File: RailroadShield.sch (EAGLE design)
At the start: 39 parts, among them J1 I2C, J4 MST4V, J5 RJ12, J6 RJ12, Q1 2N3904, U1 LM393N, U2 MCP2515-P, U3 MCP2551-P, Y1 RESONATORPTH

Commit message: 1.1
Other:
- note added: "1.1"
- note removed: "1.0"
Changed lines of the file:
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@@
 <text x="43.18" y="149.86" size="1.27" layer="250">Termination</text>
 <text x="149.86" y="27.94" size="5.08" layer="250">Locoduino</text>
-<text x="238.76" y="7.62" size="2.54" layer="250">1.0</text>
+<text x="238.76" y="7.62" size="2.54" layer="250">1.1</text>
 <text x="155.194" y="24.13" size="2.54" layer="250">Control Point</text>
 <text x="195.58" y="27.94" size="2.54" layer="250">Loconet &amp; CAN/NMRAnet</text>

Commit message: 1.2
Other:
- note added: "1.2"
- note removed: "1.1"
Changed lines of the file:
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@@
 <text x="43.18" y="149.86" size="1.27" layer="250">Termination</text>
 <text x="149.86" y="27.94" size="5.08" layer="250">Locoduino</text>
-<text x="238.76" y="7.62" size="2.54" layer="250">1.1</text>
+<text x="238.76" y="7.62" size="2.54" layer="250">1.2</text>
 <text x="155.194" y="24.13" size="2.54" layer="250">Control Point</text>
 <text x="195.58" y="27.94" size="2.54" layer="250">Loconet &amp; CAN/NMRAnet</text>

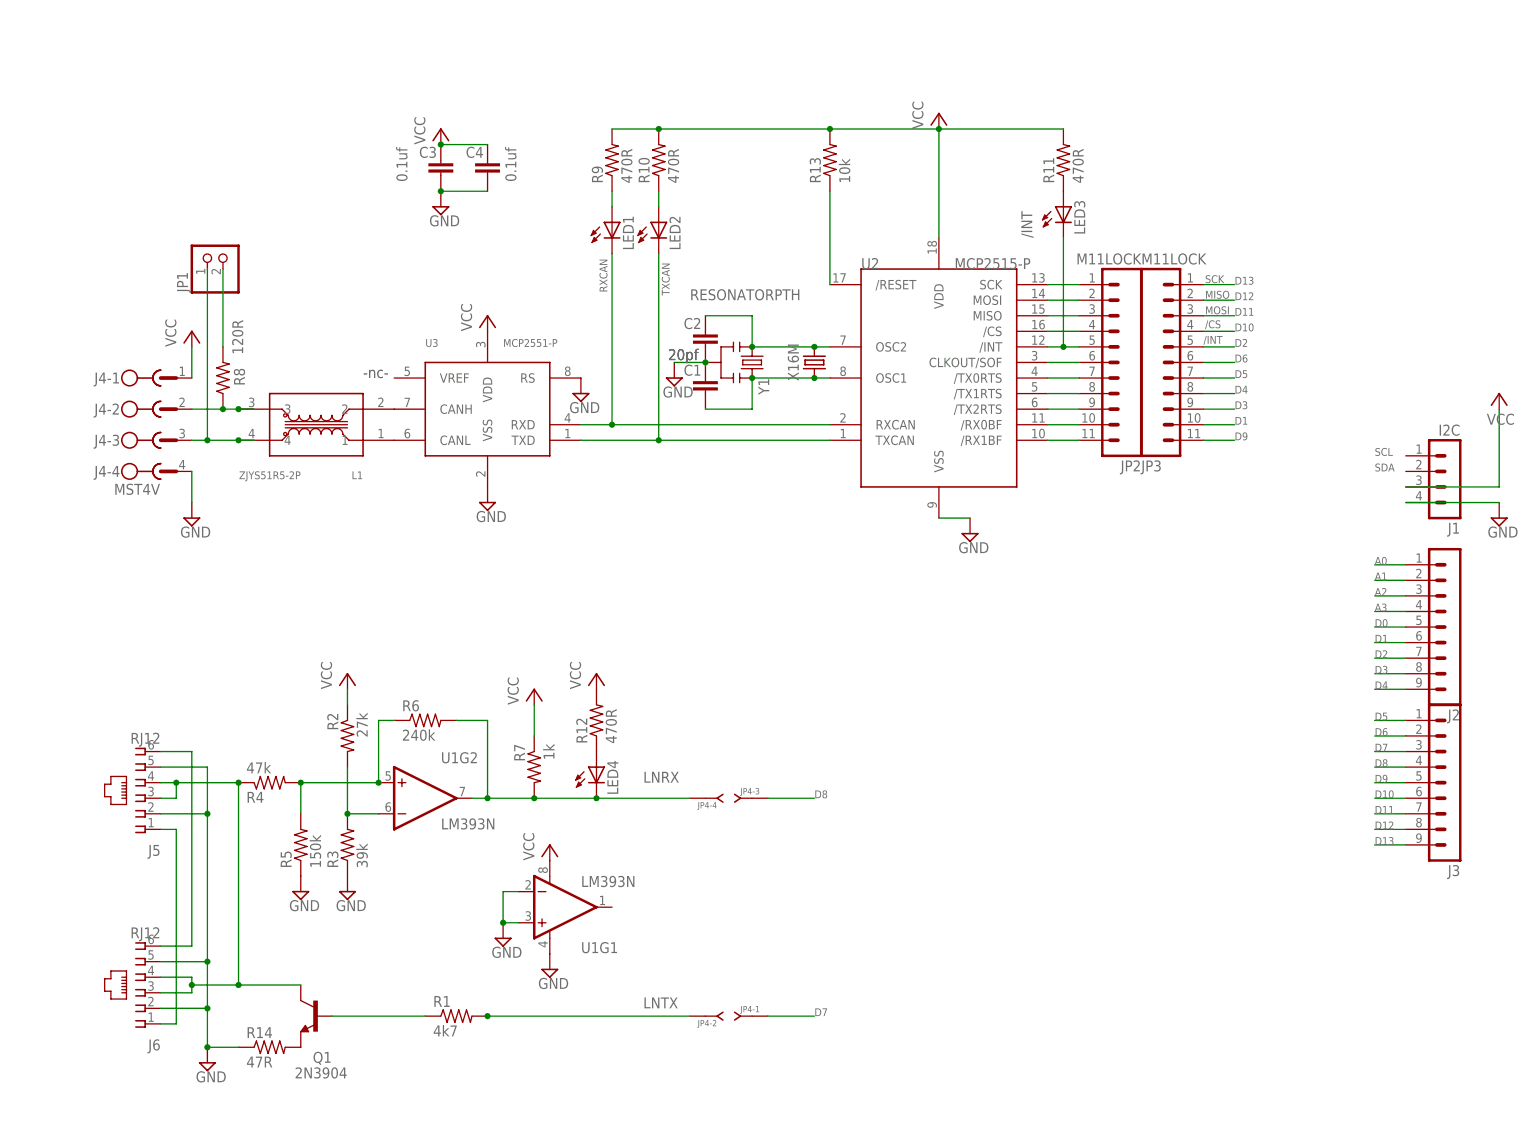
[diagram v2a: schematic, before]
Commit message: 1.3
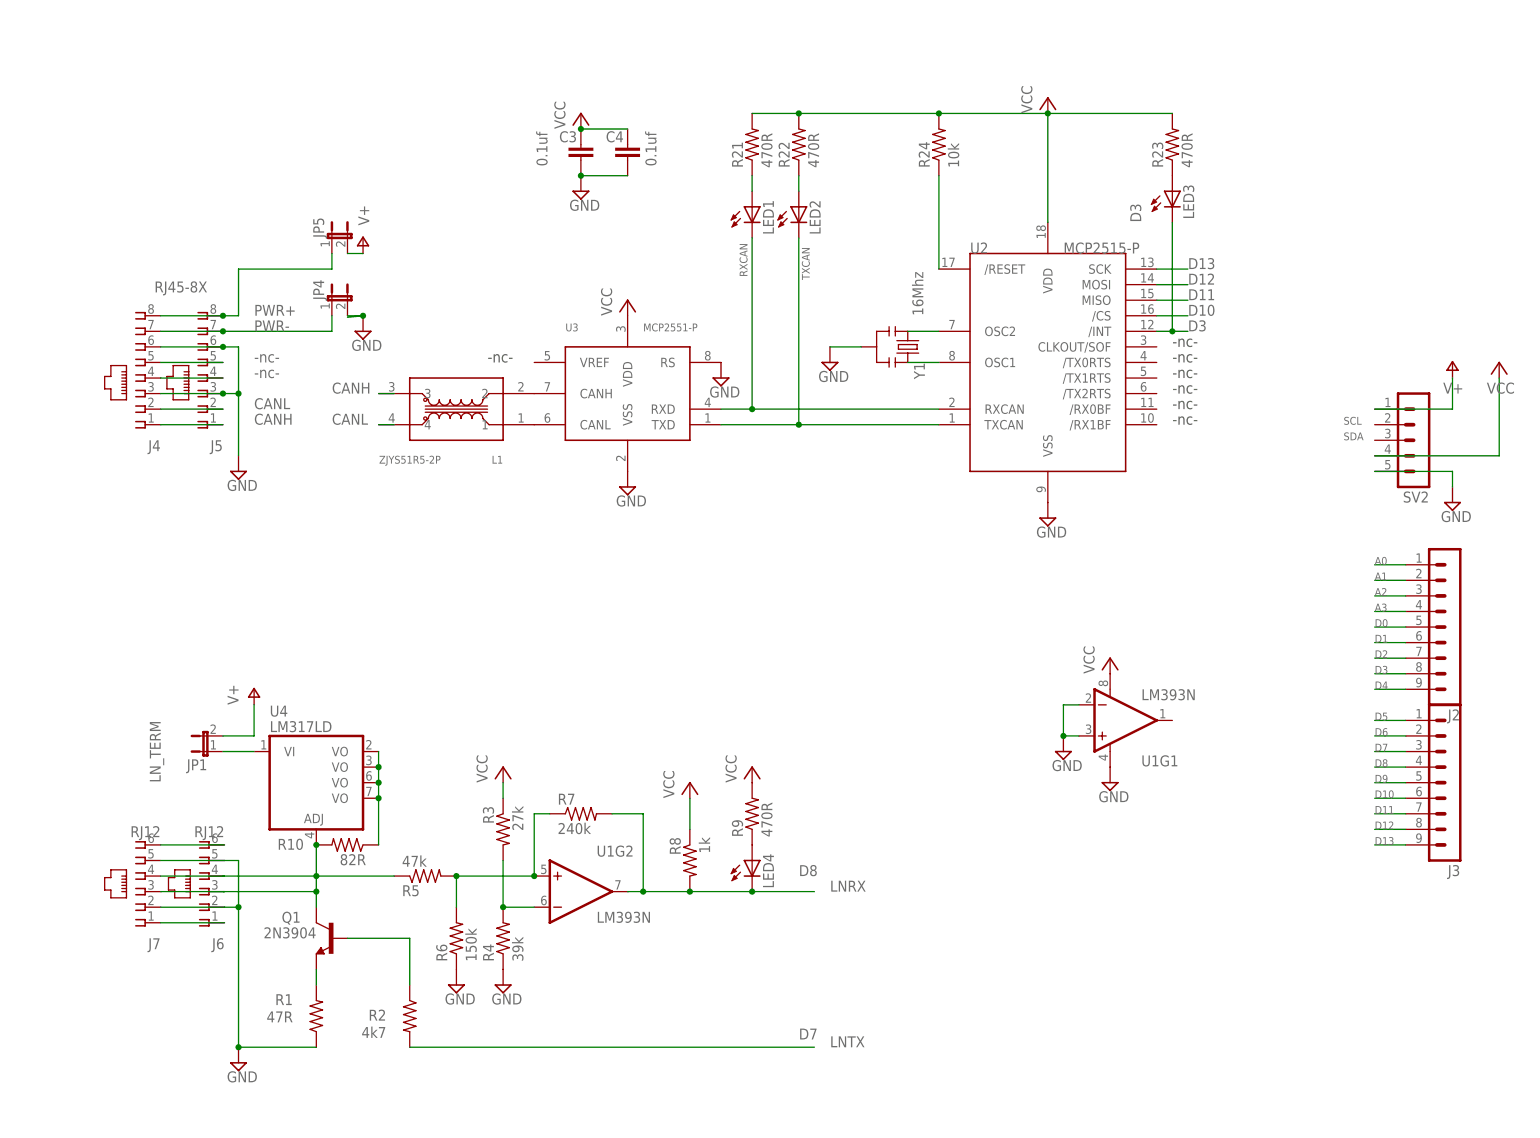
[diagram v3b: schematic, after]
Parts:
- removed C1, C2: 20pf, SparkFun:CAP0603-CAP
- removed J1: I2C, con-lstb:MA04-1
- removed JP2, JP3: M11LOCK, SparkFun:M11LOCK
- removed R11, R12: 470R, rcl:R-US_R1206W
- removed R13: 10k, rcl:R-US_R1206W
- removed R14: 47R, rcl:R-US_R1206W
- removed X16M: (no value), crystal:CRYSTALHC49S
- added J7: RJ12, con-amp:520250-3
- added JP5: (no value), SparkFun:JUMPER-2PTH_LOCK
- added R21, R22, R23: 470R, rcl:R-US_R1206W
- added R24: 10k, rcl:R-US_R1206W
- added SV2: (no value), con-lstb:MA05-1
- added U4: LM317LD, linear:LM317LD
- J4: value MST4V -> RJ45-8X; device con-phoenix-508:MST4V -> con-tycoelectronics:RJ45-8X
- J5: value RJ12 -> RJ45-8X; device con-amp:520250-3 -> con-tycoelectronics:RJ45-8X
- JP1: device pinhead:PINHD-1X2 -> SparkFun:JUMPER-2PTH
- JP4: value J-04-100-2X02 -> (none); device con-headers-jp:J-04-100-2X02 -> SparkFun:JUMPER-2PTH_LOCK
- R1: value 4k7 -> 47R
- R10: value 470R -> 82R
- R2: value 27k -> 4k7
- R3: value 39k -> 27k
- R4: value 47k -> 39k
- R5: value 150k -> 47k
- R6: value 240k -> 150k
- R7: value 1k -> 240k
- R8: value 120R -> 1k
- Y1: value RESONATORPTH -> 16Mhz
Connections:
- removed net /INT: JP2.5, LED3.C, U2./INT
- removed net /RX0BF: JP2.10, U2./RX0BF
- removed net /RX1BF: JP2.11, U2./RX1BF
- removed net /TX0RTS: JP2.7, U2./TX0RTS
- removed net /TX1RTS: JP2.8, U2./TX1RTS
- removed net /TX2RTS: JP2.9, U2./TX2RTS
- removed net CLKOUT: JP2.6, U2.CLKOUT/SOF
- removed net DCCRAILSYNC-: J5.1, J6.1
- removed net LNRX: JP4-4.J, LED4.C, R6.2, R7.2, U1G2.OUT
- removed net LNTX: JP4-2.J, R1.2
- removed net N$20: JP2.4, U2./CS
- removed net OSC2: C2.1, U2.OSC2, X16M.2, Y1.1
- removed net RAILSYNC+: J5.6, J6.6
- new net CANH: J4.1, J5.1, L1.3
- new net CANL: J4.2, J5.2, L1.4
- new net N$17: R10.1, U4.VO, U4.VO@1, U4.VO@2, U4.VO@3
- new net N$18: J4.4, J5.4
- new net N$21: J4.5, J5.5
- new net PWR+: J4.8, J5.8, JP5.1
- new net PWR-: J4.7, J5.7, JP4.1
- new net V+: JP1.2, JP5.2, SV2.1
- net /RESET: now also R24.1; no longer R13.1
- net D1: no longer JP3.10
- net D10: now also U2./CS; no longer JP3.4
- net D11: now also U2.MISO; no longer JP3.3
- net D12: now also U2.MOSI; no longer JP3.2
- net D13: now also U2.SCK; no longer JP3.1
- net D2: no longer JP3.5
- net D3: now also LED3.C, U2./INT; no longer JP3.9
- net D4: no longer JP3.8
- net D5: no longer JP3.7
- net D6: no longer JP3.6
- net D7: now also R2.2; no longer JP4-1.J
- net D8: now also LED4.C, R7.2, R8.2, U1G2.OUT; no longer JP4-3.J
- net D9: no longer JP3.11
- net GND: now also J4.3, J4.6, J5.3, J5.6, J7.2, J7.5, JP4.2, R1.1, R4.1, R6.1, SV2.5; no longer C1.1, C2.2, J1.4, J4-4.1, J5.2, J5.5, R14.1, R3.1, R5.1
- net LOCONET: now also R10.2, R5.1, U4.ADJ; no longer J5.3, J5.4, J6.3, J6.4, R4.1
- net N$1: now also R2.1; no longer R1.1
- net N$10: now also J6.6, J7.6; no longer JP1.2, R8.2
- net N$11: now also R21.1; no longer R9.1
- net N$12: now also R22.1; no longer R10.1
- net N$13: now also J6.3, J7.3; no longer JP2.1, U2.SCK
- net N$14: now also R23.1; no longer R11.1
- net N$15: now also R9.1; no longer R12.1
- net N$16: now also J6.4, J7.4; no longer JP2.2, U2.MOSI
- net N$19: now also JP1.1, U4.VI; no longer JP2.3, U2.MISO
- net N$2: now also R6.2, R7.1; no longer R4.2, R6.1
- net N$5: now also R4.2; no longer R2.2
- net N$6: now also R1.2; no longer R14.2
- net N$8: now also U2.OSC2, Y1.1; no longer J4-2.1, L1.3, R8.1
- net N$9: now also J6.1, J7.1; no longer J4-3.1, JP1.1, L1.4
- net OSC1: no longer C1.2, X16M.1
- net VCC: now also R21.2, R22.2, R23.2, R24.2, R3.1, R8.1, SV2.4; no longer J1.3, J4-1.1, R10.2, R11.2, R12.2, R13.2, R2.1, R7.1
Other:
- note added: "1.3"
- note added: "LNRX"
- note added: "LNTX"
- note added: "LN_TERM"
- note removed: "/CS"
- note removed: "/INT"
- note removed: "1.2"
- note removed: "MISO"
- note removed: "MOSI"
- note removed: "SCK"
- note removed: "Termination"
- moved on the sheet: C3, C4, J6, L1, LED1, LED2, LED3, LED4, Q1, R1, R10, R2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

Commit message: 2.0
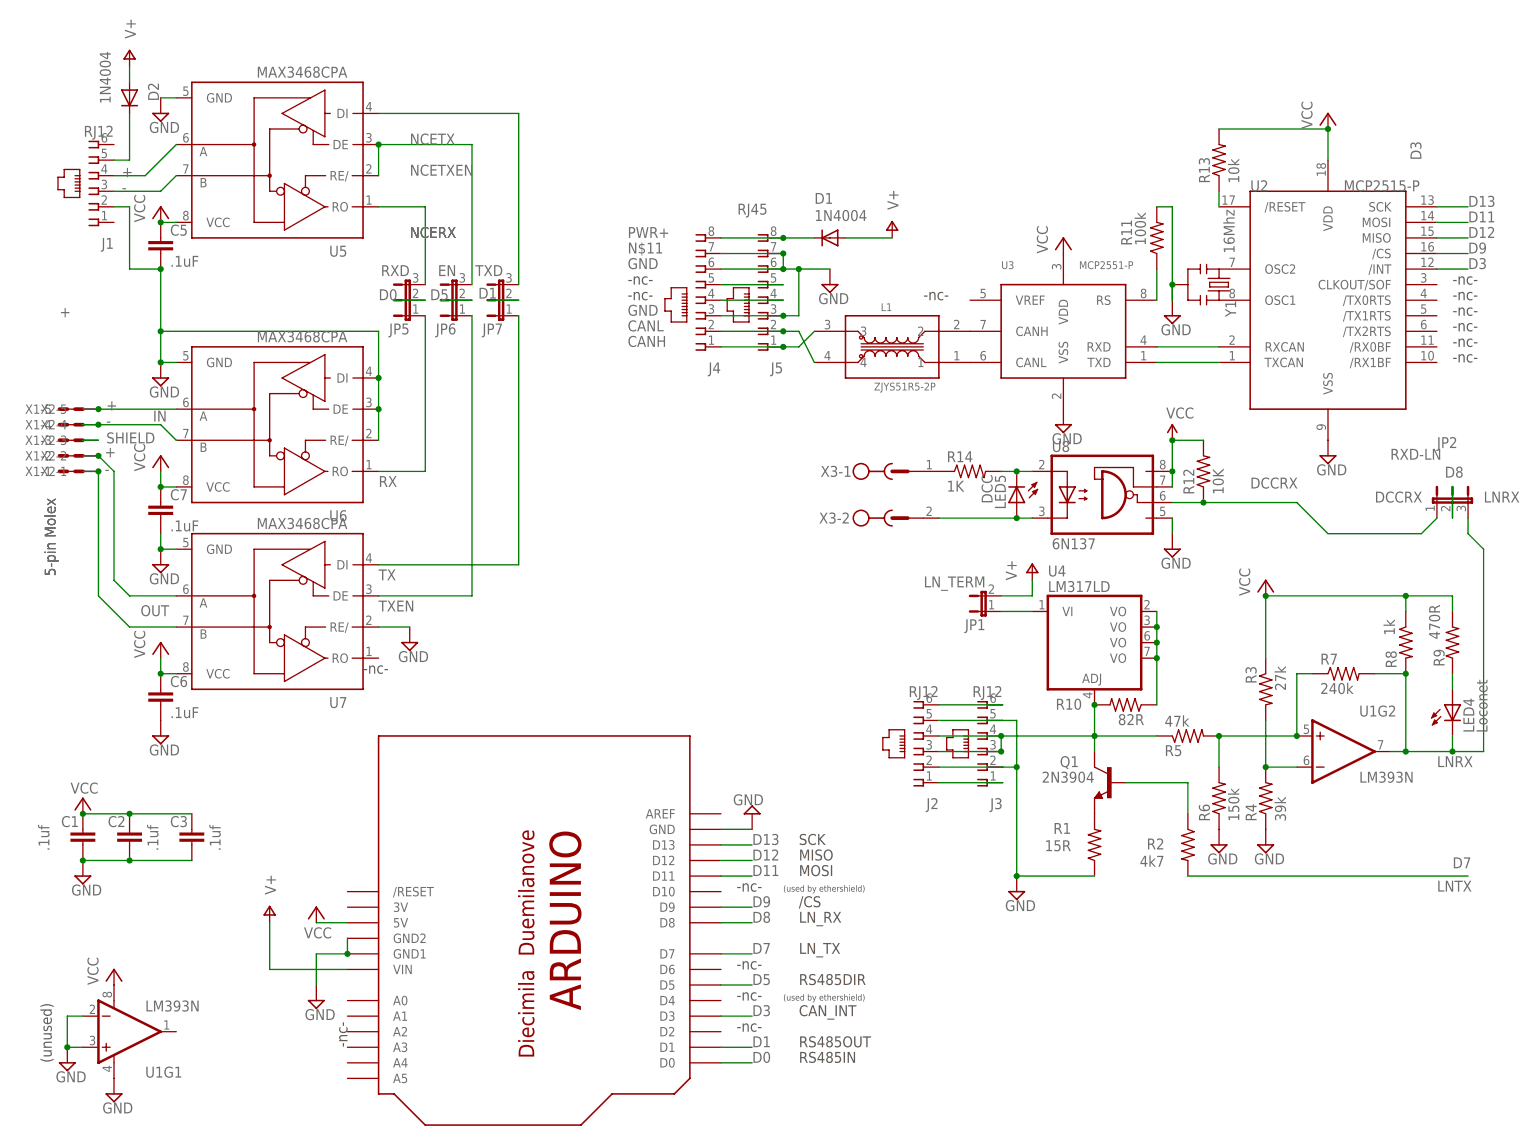
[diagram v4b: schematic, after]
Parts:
- removed C4: 0.1uf, SparkFun:CAPPTH2
- removed J6, J7: RJ12, con-amp:520250-3
- removed JP4: (no value), SparkFun:JUMPER-2PTH_LOCK
- removed LED1, LED2, LED3: (no value), MCP:LEDB155
- removed R21, R22, R23: 470R, rcl:R-US_R1206W
- removed R24: 10k, rcl:R-US_R1206W
- removed SV2: (no value), con-lstb:MA05-1
- added C1, C2: .1uf, SparkFun:CAPPTH2
- added C5, C6, C7: .1uF, SparkFun:CAPPTH2
- added D1, D2: 1N4004, diode:1N4004
- added J1: RJ12, con-amp:520250-3
- added JP2: RXD-LN, SparkFun:JUMPER-3PTH
- added JP6: EN, SparkFun:JUMPER-3PTH
- added JP7: TXD, SparkFun:JUMPER-3PTH
- added LED5: DCC, MCP:LEDCHIP-LED0805
- added MOD1: ARDUINO DUEMILANOVE, microbuilder:ARDUINODUEMILANOVE
- added R11: 100k, rcl:R-US_R1206
- added R12: 10K, SparkFun:RESISTOR1206
- added R13: 10k, rcl:R-US_R1206
- added R14: 1K, SparkFun:RESISTOR1206
- added U5, U6, U7: MAX3468CPA, maxim:MAX3468CPA
- added U8: 6N137, optocoupler:6N137
- added X1, X2: 5-pin Molex, con-molex:KK-156-5
- added X3: (no value), con-phoenix-500:MSTBV2
- C3: value 0.1uf -> .1uf
- J2, J3: value (none) -> RJ12; device con-lstb:MA09-1 -> con-amp:520250-3
- J4, J5: value RJ45-8X -> RJ45
- JP1: value (none) -> LN_TERM
- JP5: value (none) -> RXD; device SparkFun:JUMPER-2PTH_LOCK -> SparkFun:JUMPER-3PTH
- LED4: value (none) -> Loconet; device MCP:LEDB155 -> MCP:LEDCHIP-LED0805
- R1: value 47R -> 15R; device rcl:R-US_R1206W -> rcl:R-US_R1206
- R10, R2, R3, R4, R5, R6, R7, R8, R9: device rcl:R-US_R1206W -> rcl:R-US_R1206
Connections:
- removed net A0: J2.1
- removed net A1: J2.2
- removed net A2: J2.3
- removed net A3: J2.4
- removed net D10: J3.6, U2./CS
- removed net D2: J2.7
- removed net D4: J2.9
- removed net D6: J3.2
- removed net N$12: LED2.A, R22.1
- removed net N$14: LED3.A, R23.1
- removed net PWR-: J4.7, J5.7, JP4.1
- new net -OUT+: U7.B, X1-1.S, X2-1.S
- new net CMRIRX: JP5.1, U6.RO
- new net CMRITX: JP7.1, U7.DI
- new net CMRITXEN: JP6.1, U7.DE
- new net DCCRX: JP2.1, R12.1, U8.VO
- new net IN+: U6.A, X1-5.S, X2-5.S
- new net IN-: U6.B, X1-4.S, X2-4.S
- new net LNRX: JP2.3, LED4.C, R7.2, R8.2, U1G2.OUT
- new net N$20: R14.1, X3-1.SK
- new net N$23: J2.3, J3.3
- new net N$24: J1.4, U5.A
- new net N$25: J1.3, U5.B
- new net N$26: D2.C, J1.5
- new net N$4: R11.1, U3.RS
- new net NCERX: JP5.3, U5.RO
- new net NCETX: JP7.3, U5.DI
- new net NCETXEN: JP6.3, U5.DE, U5.RE/
- new net OUT+: U7.A, X1-2.S, X2-2.S
- new net SHIELD: X1-3.S, X2-3.S
- net /RESET: now also R13.1; no longer R24.1
- net D0: now also JP5.2, MOD1.D0; no longer J2.5
- net D1: now also JP7.2, MOD1.D1; no longer J2.6
- net D11: now also MOD1.D11, U2.MOSI; no longer J3.7, U2.MISO
- net D12: now also MOD1.D12, U2.MISO; no longer J3.8, U2.MOSI
- net D13: now also MOD1.D13; no longer J3.9
- net D3: now also MOD1.D3; no longer J2.8, LED3.C
- net D5: now also JP6.2, MOD1.D5; no longer J3.1
- net D7: now also MOD1.D7; no longer J3.3
- net D8: now also JP2.2, MOD1.D8; no longer J3.4, LED4.C, R7.2, R8.2, U1G2.OUT
- net D9: now also MOD1.D9, U2./CS; no longer J3.5
- net GND: now also C1.2, C2.2, C5.2, C6.2, C7.2, J1.2, J2.2, J2.5, J3.2, J3.5, MOD1.GND, MOD1.GND1, MOD1.GND2, R11.2, U5.GND, U6.DE, U6.DI, U6.GND, U6.RE/, U7.GND, U7.RE/, U8.GND; no longer C4.2, J6.2, J6.5, J7.2, J7.5, JP4.2, SV2.5, U3.RS
- net LOCONET: now also J2.4, J3.4
- net N$10: now also J2.6, J3.6; no longer J6.6, J7.6
- net N$11: now also J4.7, J5.7; no longer LED1.A, R21.1
- net N$13: now also LED5.A, U8.C, X3-2.SK; no longer J6.3, J7.3
- net N$16: now also LED5.C, R14.2, U8.A; no longer J6.4, J7.4
- net N$9: now also J2.1, J3.1; no longer J6.1, J7.1
- net PWR+: now also D1.C; no longer JP5.1
- net RXCAN: no longer LED1.C
- net TXCAN: no longer LED2.C
- net V+: now also D1.A, D2.A, MOD1.VIN; no longer JP5.2, SV2.1
- net VCC: now also C1.1, C2.1, C5.1, C6.1, C7.1, MOD1.5V, R12.2, R13.2, U5.VCC, U6.VCC, U7.VCC, U8.VCC, U8.VE; no longer C4.1, R21.2, R22.2, R23.2, R24.2, SV2.4
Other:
- note added: "(unused)"
- note added: "(used by ethershield)"
- note added: "+"
- note added: "-"
- note added: "/CS"
- note added: "2.0"
- note added: "C/MRI RS485 HD"
- note added: "C/MRI, NCE, XPressNet"
- note added: "CAN_INT"
- note added: "DCC"
- note added: "IN"
- note added: "LN_RX"
- note added: "LN_TX"
- note added: "Loconet, CAN/openLCB"
- note added: "MISO"
- note added: "MOSI"
- note added: "NCE Cab Bus Interface"
- note added: "OUT"
- note added: "RS485DIR"
- note added: "RS485IN"
- note added: "RS485OUT"
- note added: "RX"
- note added: "SCK"
- note added: "SHIELD"
- note added: "TX"
- note added: "TXEN"
- note added: "and DCC interface board"
- note added: "openLCB CAN Interface"
- note removed: "1.3"
- note removed: "LNRX"
- note removed: "LN_TERM"
- note removed: "Loconet & CAN/NMRAnet"
- note removed: "NMRAnet CAN Interface"
- note removed: "SCL"
- note removed: "SDA"
- moved on the sheet: C3, J4, J5, JP1, L1, LED4, Q1, R1, R10, R2, R3, R4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
